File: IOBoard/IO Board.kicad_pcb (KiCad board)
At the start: 2 copper layers, 103.8 x 135.5 mm, 28 parts, among them J1 Conn_01x04_Male, J2 Conn_01x04_Male, U1 AP2112K-3.3, U2 ATSAMD09D14A-M, U3 ATSAMD09D14A-M

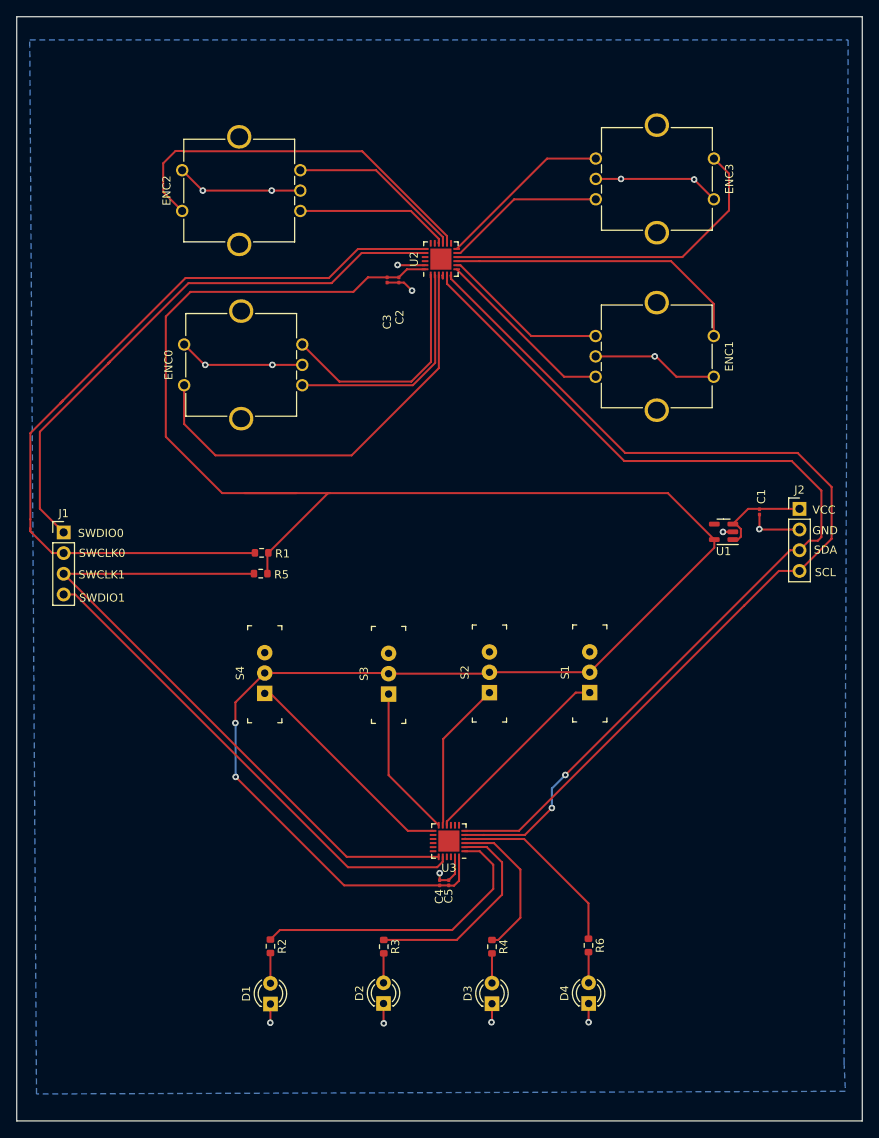
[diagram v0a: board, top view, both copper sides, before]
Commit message: Revert "Revert "Merge remote-tracking branch 'upstream/main'""
This reverts commit 1d57ca07421005fad3c6f783a10b39dbb3c17bbf.
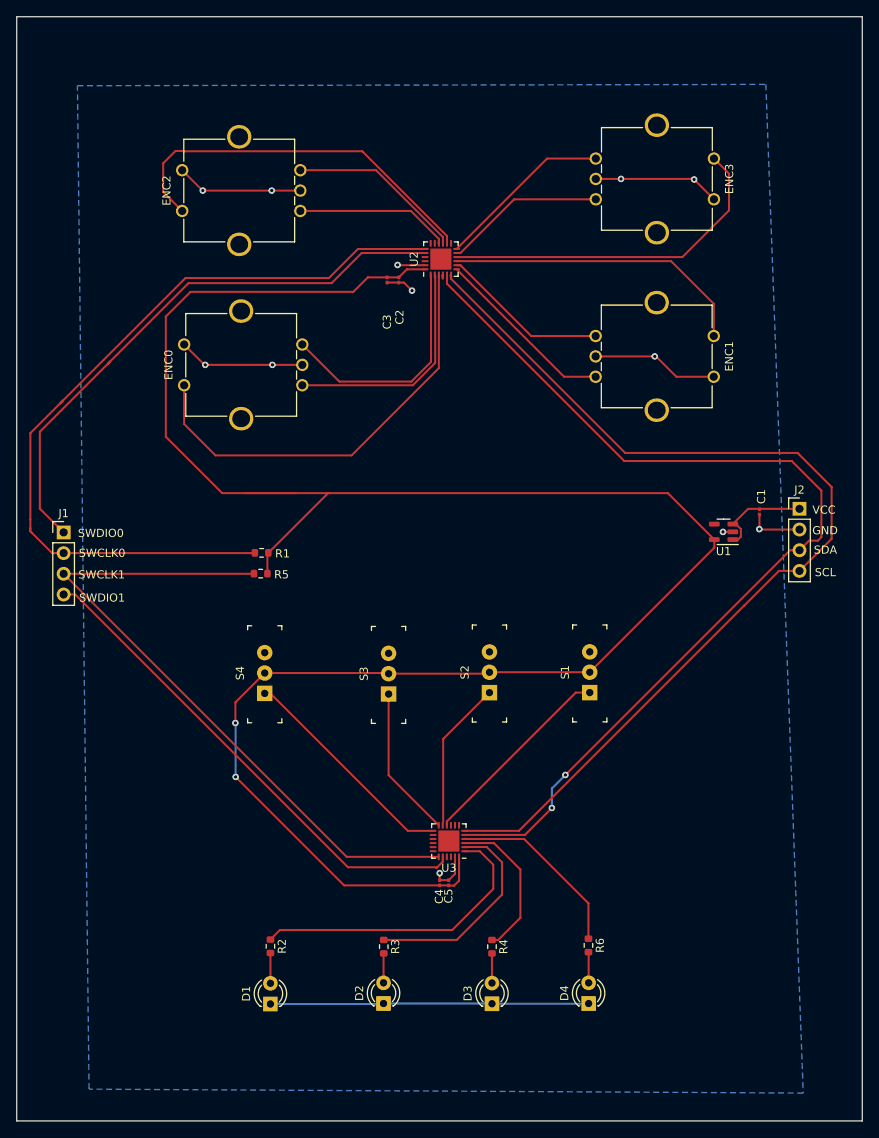
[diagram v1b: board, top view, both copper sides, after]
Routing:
- net GND: track 91.6 -> 121.2 mm, vias 17 -> 13
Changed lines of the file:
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@@
   (segment (start 138.4725 55.71) (end 135.12 55.71) (width 0.25) (layer "F.Cu") (net 2))
   (segment (start 142.14 128.3175) (end 142.14 130.41) (width 0.25) (layer "F.Cu") (net 2))
-  (segment (start 133.37 148.72) (end 133.4 148.75) (width 0.25) (layer "F.Cu") (net 2))
   (segment (start 179.51 88.08) (end 179.49 88.1) (width 0.25) (layer "F.Cu") (net 2))
   (segment (start 108.9 65.44) (end 111.4 67.94) (width 0.25) (layer "F.Cu") (net 2))
@@
   (segment (start 179.54 88.15) (end 179.49 88.1) (width 0.25) (layer "F.Cu") (net 2))
   (segment (start 119.73 67.94) (end 123.4 67.94) (width 0.25) (layer "F.Cu") (net 2))
-  (segment (start 133.37 146.32) (end 133.37 148.72) (width 0.25) (layer "F.Cu") (net 2))
-  (segment (start 119.49 148.66) (end 119.47 148.68) (width 0.25) (layer "F.Cu") (net 2))
   (segment (start 175.04 88.43) (end 175.03 88.44) (width 0.25) (layer "F.Cu") (net 2))
   (segment (start 159.42 45.12) (end 162.52 45.12) (width 0.25) (layer "F.Cu") (net 2))
@@
   (segment (start 135.25 57.84) (end 135.88 57.84) (width 0.25) (layer "F.Cu") (net 2))
   (segment (start 135.88 57.84) (end 136.87 58.83) (width 0.25) (layer "F.Cu") (net 2))
-  (segment (start 119.49 146.38) (end 119.49 148.66) (width 0.25) (layer "F.Cu") (net 2))
   (segment (start 119.65 46.55) (end 111.19 46.55) (width 0.25) (layer "F.Cu") (net 2))
   (segment (start 140.26 131.18) (end 140.26 130.32) (width 0.25) (layer "F.Cu") (net 2))
-  (segment (start 146.68 148.56) (end 146.62 148.62) (width 0.25) (layer "F.Cu") (net 2))
   (segment (start 166.81 66.9) (end 169.31 69.4) (width 0.25) (layer "F.Cu") (net 2))
   (segment (start 171.49 45.19) (end 173.92 47.62) (width 0.25) (layer "F.Cu") (net 2))
@@
   (segment (start 135.12 55.71) (end 135.09 55.68) (width 0.25) (layer "F.Cu") (net 2))
   (segment (start 176.24 88.43) (end 175.04 88.43) (width 0.25) (layer "F.Cu") (net 2))
-  (segment (start 158.54 146.32) (end 158.54 148.62) (width 0.25) (layer "F.Cu") (net 2))
   (segment (start 111.19 46.55) (end 111.16 46.55) (width 0.25) (layer "F.Cu") (net 2))
   (segment (start 179.51 86.305) (end 179.51 88.08) (width 0.25) (layer "F.Cu") (net 2))
   (segment (start 111.4 67.94) (end 111.49 67.94) (width 0.25) (layer "F.Cu") (net 2))
   (segment (start 141.37 131.18) (end 140.26 131.18) (width 0.25) (layer "F.Cu") (net 2))
-  (segment (start 146.68 146.35) (end 146.68 148.56) (width 0.25) (layer "F.Cu") (net 2))
-  (via (at 133.4 148.75) (size 0.8) (drill 0.4) (layers "F.Cu" "B.Cu") (net 2))
   (via (at 179.49 88.1) (size 0.8) (drill 0.4) (layers "F.Cu" "B.Cu") (net 2))
   (via (at 123.4 67.94) (size 0.8) (drill 0.4) (layers "F.Cu" "B.Cu") (net 2))
-  (via (at 119.47 148.68) (size 0.8) (drill 0.4) (layers "F.Cu" "B.Cu") (net 2))
   (via (at 136.87 58.83) (size 0.8) (drill 0.4) (layers "F.Cu" "B.Cu") (net 2))
   (via (at 166.66 66.9) (size 0.8) (drill 0.4) (layers "F.Cu" "B.Cu") (net 2))
@@
   (via (at 111.19 46.55) (size 0.8) (drill 0.4) (layers "F.Cu" "B.Cu") (net 2))
   (via (at 111.49 67.94) (size 0.8) (drill 0.4) (layers "F.Cu" "B.Cu") (net 2))
-  (via (at 158.54 148.62) (size 0.8) (drill 0.4) (layers "F.Cu" "B.Cu") (net 2))
   (via (at 119.65 46.55) (size 0.8) (drill 0.4) (layers "F.Cu" "B.Cu") (net 2))
   (via (at 171.49 45.19) (size 0.8) (drill 0.4) (layers "F.Cu" "B.Cu") (net 2))
@@
   (via (at 119.73 67.94) (size 0.8) (drill 0.4) (layers "F.Cu" "B.Cu") (net 2))
   (via (at 140.26 130.32) (size 0.8) (drill 0.4) (layers "F.Cu" "B.Cu") (net 2))
-  (via (at 146.62 148.62) (size 0.8) (drill 0.4) (layers "F.Cu" "B.Cu") (net 2))
+  (segment (start 146.68 146.35) (end 158.51 146.35) (width 0.25) (layer "B.Cu") (net 2))
+  (segment (start 133.37 146.32) (end 146.65 146.32) (width 0.25) (layer "B.Cu") (net 2))
   (segment (start 158.51 146.35) (end 158.54 146.32) (width 0.25) (layer "B.Cu") (net 2))
   (segment (start 146.65 146.32) (end 146.68 146.35) (width 0.25) (layer "B.Cu") (net 2))
+  (segment (start 119.49 146.38) (end 133.31 146.38) (width 0.25) (layer "B.Cu") (net 2))
   (segment (start 133.31 146.38) (end 133.37 146.32) (width 0.25) (layer "B.Cu") (net 2))
   (segment (start 115.19 111.89) (end 115.19 109.36) (width 0.25) (layer "F.Cu") (net 3))
@@
   (segment (start 99.09 93.58) (end 99.16 93.65) (width 0.25) (layer "F.Cu") (net 21))
   (segment (start 94.11 93.58) (end 99.09 93.58) (width 0.25) (layer "F.Cu") (net 21))
+  (segment (start 139.957348 129.597348) (end 139.844695 129.71) (width 0.25) (layer "F.Cu") (net 22))
   (segment (start 129.007348 129.597348) (end 95.53 96.12) (width 0.25) (layer "F.Cu") (net 22))
   (segment (start 139.957348 129.597348) (end 129.007348 129.597348) (width 0.25) (layer "F.Cu") (net 22))
@@
   (segment (start 140.610996 57.309004) (end 140.610996 56.946504) (width 0.25) (layer "F.Cu") (net 53))
   (segment (start 140.66 57.358008) (end 140.66 56.8975) (width 0.25) (layer "F.Cu") (net 53))
+  (zone (net 0) (net_name "") (layer "B.Cu") (hatch edge 0.508)
+    (connect_pads (clearance 0))
+    (min_thickness 0.254)
+    (keepout (tracks allowed) (vias allowed) (pads not_allowed) (copperpour not_allowed) (footprints allowed))
+    (fill (thermal_gap 0.508) (thermal_bridge_width 0.508))
+    (polygon
+      (pts
+        (xy 121.97 119.17)
+        (xy 112.53 119.2)
+        (xy 112.5 111.16)
+        (xy 121.31 111.09)
+      )
+    )
+  )
+  (zone (net 0) (net_name "") (layer "B.Cu") (hatch edge 0.508)
+    (connect_pads (clearance 0))
+    (min_thickness 0.254)
+    (keepout (tracks allowed) (vias allowed) (pads not_allowed) (copperpour allowed) (footprints allowed))
+    (fill (thermal_gap 0.508) (thermal_bridge_width 0.508))
+    (polygon
+      (pts
+        (xy 161.82 123.31)
+        (xy 152.51 123.61)
+        (xy 152.57 117.34)
+        (xy 161.79 117.13)
+      )
+    )
+  )
   (zone (net 2) (net_name "GND") (layer "B.Cu") (hatch edge 0.508)
     (connect_pads (clearance 0.508))
-    (min_thickness 0.254) (filled_areas_thickness no)
-    (fill yes (thermal_gap 0.508) (thermal_bridge_width 0.508))
+    (min_thickness 0.254)
+    (fill (thermal_gap 0.508) (thermal_bridge_width 0.508))
     (polygon
       (pts
-        (xy 189.89 153.6)
-        (xy 190.06 157.09)
-        (xy 90.78 157.42)
-        (xy 89.95 28.06)
-        (xy 190.39 28.06)
+        (xy 184.88 157.31)
+        (xy 97.23 156.83)
+        (xy 95.801852 33.679713)
+        (xy 180.29 33.52)
       )
     )

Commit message: Revert "Merge remote-tracking branch 'upstream/main'"
This reverts commit 91e618c32c18b3f8ce9c65181e2c7ed2aa69dacd, reversing
changes made to 5f9fe177db78953ec4a0d750e6893e90b3881885.
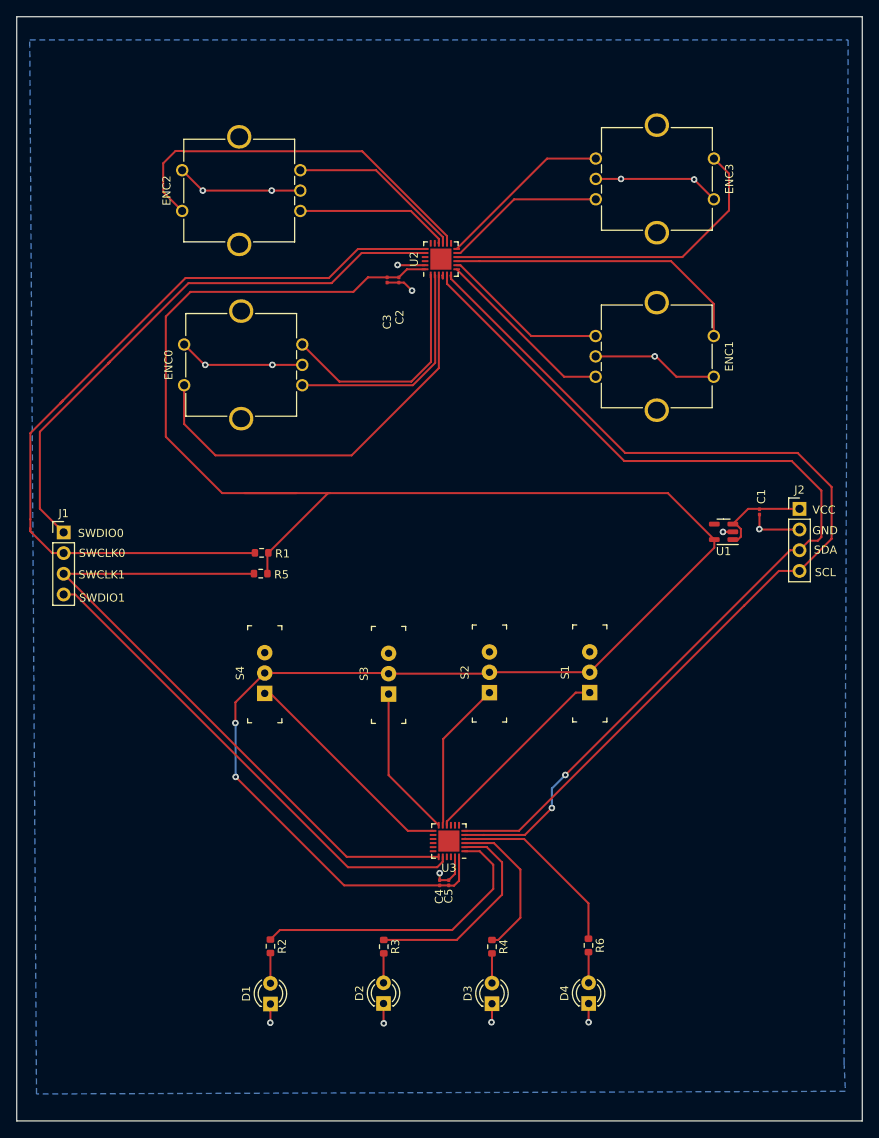
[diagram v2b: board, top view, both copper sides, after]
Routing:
- net GND: track 121.2 -> 91.6 mm, vias 13 -> 17
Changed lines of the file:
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@@
   (segment (start 138.4725 55.71) (end 135.12 55.71) (width 0.25) (layer "F.Cu") (net 2))
   (segment (start 142.14 128.3175) (end 142.14 130.41) (width 0.25) (layer "F.Cu") (net 2))
+  (segment (start 133.37 148.72) (end 133.4 148.75) (width 0.25) (layer "F.Cu") (net 2))
   (segment (start 179.51 88.08) (end 179.49 88.1) (width 0.25) (layer "F.Cu") (net 2))
   (segment (start 108.9 65.44) (end 111.4 67.94) (width 0.25) (layer "F.Cu") (net 2))
@@
   (segment (start 179.54 88.15) (end 179.49 88.1) (width 0.25) (layer "F.Cu") (net 2))
   (segment (start 119.73 67.94) (end 123.4 67.94) (width 0.25) (layer "F.Cu") (net 2))
+  (segment (start 133.37 146.32) (end 133.37 148.72) (width 0.25) (layer "F.Cu") (net 2))
+  (segment (start 119.49 148.66) (end 119.47 148.68) (width 0.25) (layer "F.Cu") (net 2))
   (segment (start 175.04 88.43) (end 175.03 88.44) (width 0.25) (layer "F.Cu") (net 2))
   (segment (start 159.42 45.12) (end 162.52 45.12) (width 0.25) (layer "F.Cu") (net 2))
@@
   (segment (start 135.25 57.84) (end 135.88 57.84) (width 0.25) (layer "F.Cu") (net 2))
   (segment (start 135.88 57.84) (end 136.87 58.83) (width 0.25) (layer "F.Cu") (net 2))
+  (segment (start 119.49 146.38) (end 119.49 148.66) (width 0.25) (layer "F.Cu") (net 2))
   (segment (start 119.65 46.55) (end 111.19 46.55) (width 0.25) (layer "F.Cu") (net 2))
   (segment (start 140.26 131.18) (end 140.26 130.32) (width 0.25) (layer "F.Cu") (net 2))
+  (segment (start 146.68 148.56) (end 146.62 148.62) (width 0.25) (layer "F.Cu") (net 2))
   (segment (start 166.81 66.9) (end 169.31 69.4) (width 0.25) (layer "F.Cu") (net 2))
   (segment (start 171.49 45.19) (end 173.92 47.62) (width 0.25) (layer "F.Cu") (net 2))
@@
   (segment (start 135.12 55.71) (end 135.09 55.68) (width 0.25) (layer "F.Cu") (net 2))
   (segment (start 176.24 88.43) (end 175.04 88.43) (width 0.25) (layer "F.Cu") (net 2))
+  (segment (start 158.54 146.32) (end 158.54 148.62) (width 0.25) (layer "F.Cu") (net 2))
   (segment (start 111.19 46.55) (end 111.16 46.55) (width 0.25) (layer "F.Cu") (net 2))
   (segment (start 179.51 86.305) (end 179.51 88.08) (width 0.25) (layer "F.Cu") (net 2))
   (segment (start 111.4 67.94) (end 111.49 67.94) (width 0.25) (layer "F.Cu") (net 2))
   (segment (start 141.37 131.18) (end 140.26 131.18) (width 0.25) (layer "F.Cu") (net 2))
+  (segment (start 146.68 146.35) (end 146.68 148.56) (width 0.25) (layer "F.Cu") (net 2))
+  (via (at 133.4 148.75) (size 0.8) (drill 0.4) (layers "F.Cu" "B.Cu") (net 2))
   (via (at 179.49 88.1) (size 0.8) (drill 0.4) (layers "F.Cu" "B.Cu") (net 2))
   (via (at 123.4 67.94) (size 0.8) (drill 0.4) (layers "F.Cu" "B.Cu") (net 2))
+  (via (at 119.47 148.68) (size 0.8) (drill 0.4) (layers "F.Cu" "B.Cu") (net 2))
   (via (at 136.87 58.83) (size 0.8) (drill 0.4) (layers "F.Cu" "B.Cu") (net 2))
   (via (at 166.66 66.9) (size 0.8) (drill 0.4) (layers "F.Cu" "B.Cu") (net 2))
@@
   (via (at 111.19 46.55) (size 0.8) (drill 0.4) (layers "F.Cu" "B.Cu") (net 2))
   (via (at 111.49 67.94) (size 0.8) (drill 0.4) (layers "F.Cu" "B.Cu") (net 2))
+  (via (at 158.54 148.62) (size 0.8) (drill 0.4) (layers "F.Cu" "B.Cu") (net 2))
   (via (at 119.65 46.55) (size 0.8) (drill 0.4) (layers "F.Cu" "B.Cu") (net 2))
   (via (at 171.49 45.19) (size 0.8) (drill 0.4) (layers "F.Cu" "B.Cu") (net 2))
@@
   (via (at 119.73 67.94) (size 0.8) (drill 0.4) (layers "F.Cu" "B.Cu") (net 2))
   (via (at 140.26 130.32) (size 0.8) (drill 0.4) (layers "F.Cu" "B.Cu") (net 2))
-  (segment (start 146.68 146.35) (end 158.51 146.35) (width 0.25) (layer "B.Cu") (net 2))
-  (segment (start 133.37 146.32) (end 146.65 146.32) (width 0.25) (layer "B.Cu") (net 2))
+  (via (at 146.62 148.62) (size 0.8) (drill 0.4) (layers "F.Cu" "B.Cu") (net 2))
   (segment (start 158.51 146.35) (end 158.54 146.32) (width 0.25) (layer "B.Cu") (net 2))
   (segment (start 146.65 146.32) (end 146.68 146.35) (width 0.25) (layer "B.Cu") (net 2))
-  (segment (start 119.49 146.38) (end 133.31 146.38) (width 0.25) (layer "B.Cu") (net 2))
   (segment (start 133.31 146.38) (end 133.37 146.32) (width 0.25) (layer "B.Cu") (net 2))
   (segment (start 115.19 111.89) (end 115.19 109.36) (width 0.25) (layer "F.Cu") (net 3))
@@
   (segment (start 99.09 93.58) (end 99.16 93.65) (width 0.25) (layer "F.Cu") (net 21))
   (segment (start 94.11 93.58) (end 99.09 93.58) (width 0.25) (layer "F.Cu") (net 21))
-  (segment (start 139.957348 129.597348) (end 139.844695 129.71) (width 0.25) (layer "F.Cu") (net 22))
   (segment (start 129.007348 129.597348) (end 95.53 96.12) (width 0.25) (layer "F.Cu") (net 22))
   (segment (start 139.957348 129.597348) (end 129.007348 129.597348) (width 0.25) (layer "F.Cu") (net 22))
@@
   (segment (start 140.610996 57.309004) (end 140.610996 56.946504) (width 0.25) (layer "F.Cu") (net 53))
   (segment (start 140.66 57.358008) (end 140.66 56.8975) (width 0.25) (layer "F.Cu") (net 53))
-  (zone (net 0) (net_name "") (layer "B.Cu") (hatch edge 0.508)
-    (connect_pads (clearance 0))
-    (min_thickness 0.254)
-    (keepout (tracks allowed) (vias allowed) (pads not_allowed) (copperpour not_allowed) (footprints allowed))
-    (fill (thermal_gap 0.508) (thermal_bridge_width 0.508))
+  (zone (net 2) (net_name "GND") (layer "B.Cu") (hatch edge 0.508)
+    (connect_pads (clearance 0.508))
+    (min_thickness 0.254) (filled_areas_thickness no)
+    (fill yes (thermal_gap 0.508) (thermal_bridge_width 0.508))
     (polygon
       (pts
-        (xy 121.97 119.17)
-        (xy 112.53 119.2)
-        (xy 112.5 111.16)
-        (xy 121.31 111.09)
+        (xy 189.89 153.6)
+        (xy 190.06 157.09)
+        (xy 90.78 157.42)
+        (xy 89.95 28.06)
+        (xy 190.39 28.06)
       )
     )
-  )
-  (zone (net 0) (net_name "") (layer "B.Cu") (hatch edge 0.508)
-    (connect_pads (clearance 0))
-    (min_thickness 0.254)
-    (keepout (tracks allowed) (vias allowed) (pads not_allowed) (copperpour allowed) (footprints allowed))
-    (fill (thermal_gap 0.508) (thermal_bridge_width 0.508))
-    (polygon
-      (pts
-        (xy 161.82 123.31)
-        (xy 152.51 123.61)
-        (xy 152.57 117.34)
-        (xy 161.79 117.13)
-      )
-    )
-  )
-  (zone (net 2) (net_name "GND") (layer "B.Cu") (hatch edge 0.508)
-    (connect_pads (clearance 0.508))
-    (min_thickness 0.254)
-    (fill (thermal_gap 0.508) (thermal_bridge_width 0.508))
-    (polygon
-      (pts
-        (xy 184.88 157.31)
-        (xy 97.23 156.83)
-        (xy 95.801852 33.679713)
-        (xy 180.29 33.52)
-      )
-    )
